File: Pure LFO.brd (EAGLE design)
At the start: 18.3 x 100 mm, 46 parts, among them T3 TRANS_PAIR, U1 DUAL_OPAMP, U2 QUAD_OPAMP

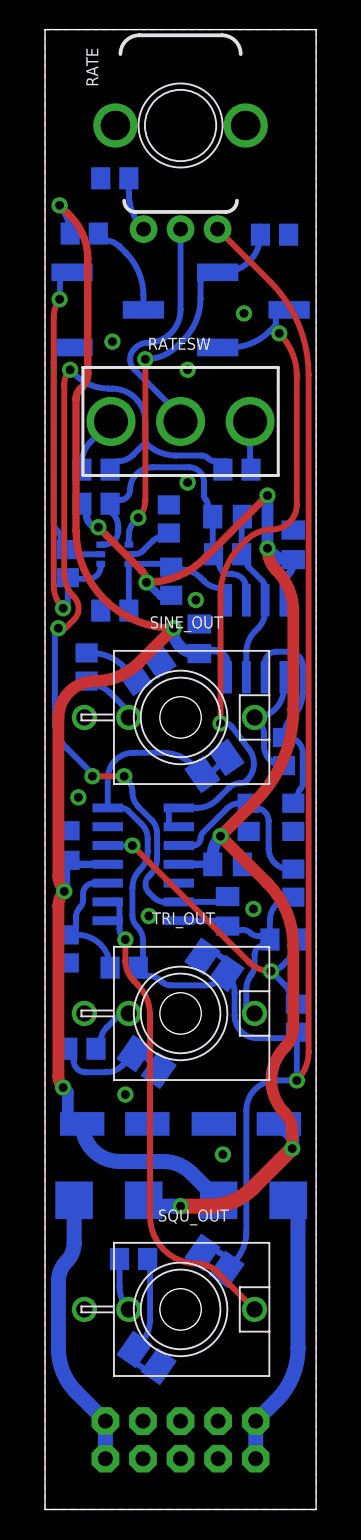
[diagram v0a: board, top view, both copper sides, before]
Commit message: LFO 2.1
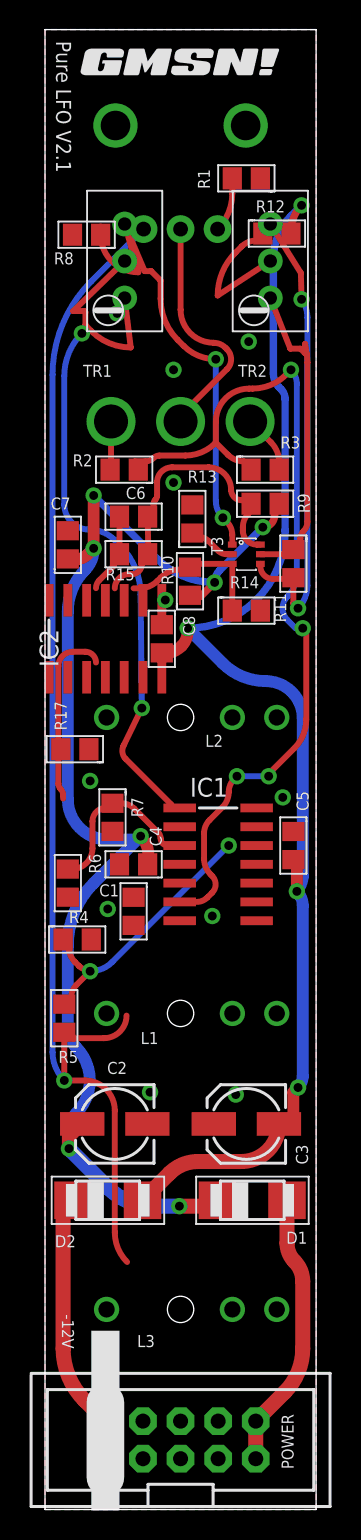
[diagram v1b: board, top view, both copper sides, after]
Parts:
- removed L1, L2, L3: (no value), INSTRUO:LSG_T77K
- removed R16: 15K, rcl:R0805
- removed R18: 50K, rcl:R0805
- removed R19: 20K, rcl:R0805
- removed R20, R21, R22: 2K*, rcl:R0805
- removed U1: DUAL_OPAMP, INSTRUO:DUAL_OPAMP
- removed U2: QUAD_OPAMP, INSTRUO:QUAD_OPAMP
- added IC1: TL074, GMSN:SO14
- added IC2: TL072, GMSN:SO14
- added U$1, U$2: (no value), gmsnLogo:GMSN!_LOGO
- C1: value 47nF -> 5n1F; device rcl:C0805K -> GMSN:C0805
- C2, C3: value 10u -> 10uF; device rcl:153CLV-0505 -> GMSN:153CLV-0505
- C4, C5, C7, C8: value 0.1u -> 100nF; device rcl:C0805K -> GMSN:C0805
- C6: device rcl:C0805K -> GMSN:C0805
- D1, D2: value (none) -> STTH102A; device adafruit:SMADIODE -> GMSN:SMADIODE
- JP1: value M05X2SHD -> HEADER2X5SHD; device SparkFun-Connectors:2X5-SHROUDED -> GMSN:2X5-SHROUDED
- R1: value 1K -> 100R; device rcl:R0805 -> GMSN:R0805
- R10, R12, R14, R15, R17, R9: value 10K -> 10k; device rcl:R0805 -> GMSN:R0805
- R11: value 400R -> 402R; device rcl:R0805 -> GMSN:R0805
- R13, R8: value 2K -> 2k; device rcl:R0805 -> GMSN:R0805
- R2: value 300R? -> 3M3; device rcl:R0805 -> GMSN:R0805
- R3: value 3M -> 3k3; device rcl:R0805 -> GMSN:R0805
- R4: value 12K -> 12k; device rcl:R0805 -> GMSN:R0805
- R5: value 33K -> 33k; device rcl:R0805 -> GMSN:R0805
- R6: value 1K3 -> 1k3; device rcl:R0805 -> GMSN:R0805
- R7: value 3K3 -> 3k3; device rcl:R0805 -> GMSN:R0805
- RATE: value B100K -> B100k; device INSTRUO:Q-POT -> GMSN:POTENTIOMETER_9MM
- RATESW: value (none) -> SWITCH_TOGGLE_SPDT; device INSTRUO:TOGGLE_ON_OFF_ON -> GMSN:TOGGLE_SW
- SINE_OUT, SQU_OUT, TRI_OUT: value (none) -> SOCKET_MONO_3.5MMPJ301M-12; device INSTRUO:S_JACK -> GMSN:PJ301M-12
- T3: value TRANS_PAIR -> DMMT3904W-7-F; device QuBit:TRANS_PAIR -> GMSN:TRANS_PAIR
- TR1: value 100K -> 100k; device INSTRUO:TRIM_3269W -> GMSN:TRIMMER_TH
- TR2: device INSTRUO:TRIM_3269W -> GMSN:TRIMMER_TH
- moved R5 15.7 mm to (2.30, 49.9), flipped to the top
- moved C5 15.2 mm to (17.8, 61.6), flipped to the top
- moved C7 15.2 mm to (2.54, 81.9), flipped to the top
- moved R11 15.2 mm to (17.8, 80.6), flipped to the top
- moved R6 15.2 mm to (2.54, 59.1), flipped to the top
- moved R17 14.1 mm to (3.02, 68.1), flipped to the top, turned to 180 degrees
- moved R4 14.0 mm to (3.17, 55.2), flipped to the top
- moved R12 13.0 mm to (16.7, 102.9), flipped to the top
- moved R8 12.7 mm to (3.81, 102.9), flipped to the top
- moved R3 11.4 mm to (15.9, 87.0), flipped to the top
- moved R9 11.4 mm to (15.9, 84.7), flipped to the top
- moved D2 9.84 mm to (5.24, 37.6), flipped to the top
- moved TR1 9.84 mm to (5.24, 97.8), flipped to the top
- moved TR2 9.84 mm to (15.1, 97.8), flipped to the top
- moved D1 9.68 mm to (15.0, 37.6), flipped to the top
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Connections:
- removed net L_SIN: R21.2, SINE_OUT.NORM
- removed net L_SQU: R20.2, SQU_OUT.NORM
- removed net L_TRI: R22.2, TRI_OUT.NORM
- removed net N$13: L1.1, L1.4, L2.1, L2.4, L3.1, L3.4, R18.1, R5.1, RATE.P$3, U2.4OUT
- removed net N$15: L1.2, L1.3, R22.1
- removed net N$16: L2.2, L2.3, R21.1
- removed net N$17: L3.2, L3.3, R20.1
- removed net SINE: R17.1, SINE_OUT.TIP, U1.1OUT
- new net SINE_WAVE: IC1.10, IC2.1, R17.1
- new net SQUARE_WAVE: IC1.14, IC2.10, R5.1, RATE.P$3
- new net TRIANGLE_WAVE: C1.2, IC1.7, IC2.12, R4.2, R6.2
- net +12V: now also IC1.4, IC2.4; no longer U1.+VCC, U2.VCC++
- net -12V: now also IC1.11, IC2.11; no longer U1.-VCC, U2.VCC--
- net GND: now also IC1.13, IC1.5; no longer R16.1, R19.1, U2.2+IN, U2.4-IN
- net N$21: now also T3.5; no longer T3.E2
- net N$25: now also T3.1; no longer T3.B2
- net N$26: now also T3.4; no longer T3.E1
- net N$28: now also T3.2; no longer T3.B1
- net N$32: now also IC2.6, T3.6; no longer T3.C2, U1.-2IN
- net N$33: now also IC1.1, IC1.2; no longer U2.1-IN, U2.1OUT
- net N$34: now also IC2.5, T3.3; no longer T3.C1, U1.+2IN
- net N$35: now also IC1.3; no longer U2.1+IN
- net N$38: now also IC2.2; no longer R16.2, U1.-1IN
- net N$5: now also IC2.8, IC2.9, SQU_OUT.TIP; no longer R18.2, R19.2, U2.3+IN
- net N$6: now also IC1.6; no longer U2.2-IN
- net N$7: now also IC2.13, IC2.14; no longer C1.2, R4.2, R6.2, U2.2OUT
- net N$8: now also IC1.8, IC1.9, SINE_OUT.TIP; no longer SQU_OUT.TIP, U2.3-IN, U2.3OUT
- net N$9: now also IC1.12; no longer U2.4+IN
- net SINE_PRE: now also IC2.3, IC2.7; no longer U1.+1IN, U1.2OUT
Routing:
- net N$13: track 123.4 -> 0.00 mm, vias 1 -> 0
- net SQUARE_WAVE: track 0.00 -> 82.6 mm, vias 0 -> 1
- net N$8: track 33.7 -> 0.00 mm, vias 1 -> 0
- net N$7: track 15.9 -> 0.00 mm
- net N$17: track 9.26 -> 0.00 mm
- net N$5: track 8.84 -> 0.00 mm
- net N$15: track 7.94 -> 0.00 mm
- net SINE: track 7.54 -> 0.00 mm
- net -12V: track 95.0 -> 88.3 mm
- net N$25: track 25.9 -> 32.3 mm
- net SINE_PRE: track 11.8 -> 5.41 mm
- net N$16: track 6.28 -> 0.00 mm
- net +12V: track 90.1 -> 84.9 mm
- net N$6: track 63.1 -> 59.2 mm
- net L_SIN: track 3.92 -> 0.00 mm
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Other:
- board text added: "-12V"
- board text added: "Pure LFO V2.1"
- board text added: "copyright GMSN Ltd 2016"
